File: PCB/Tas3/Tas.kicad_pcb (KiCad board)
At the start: 2 copper layers, 70 x 70 mm, 26 parts, among them J1 Shelly 1, J2 Conn_01x07, J3 USB-C, U1 MD8942, U2 Barcode, U3 CH340X, U4 ISL89410

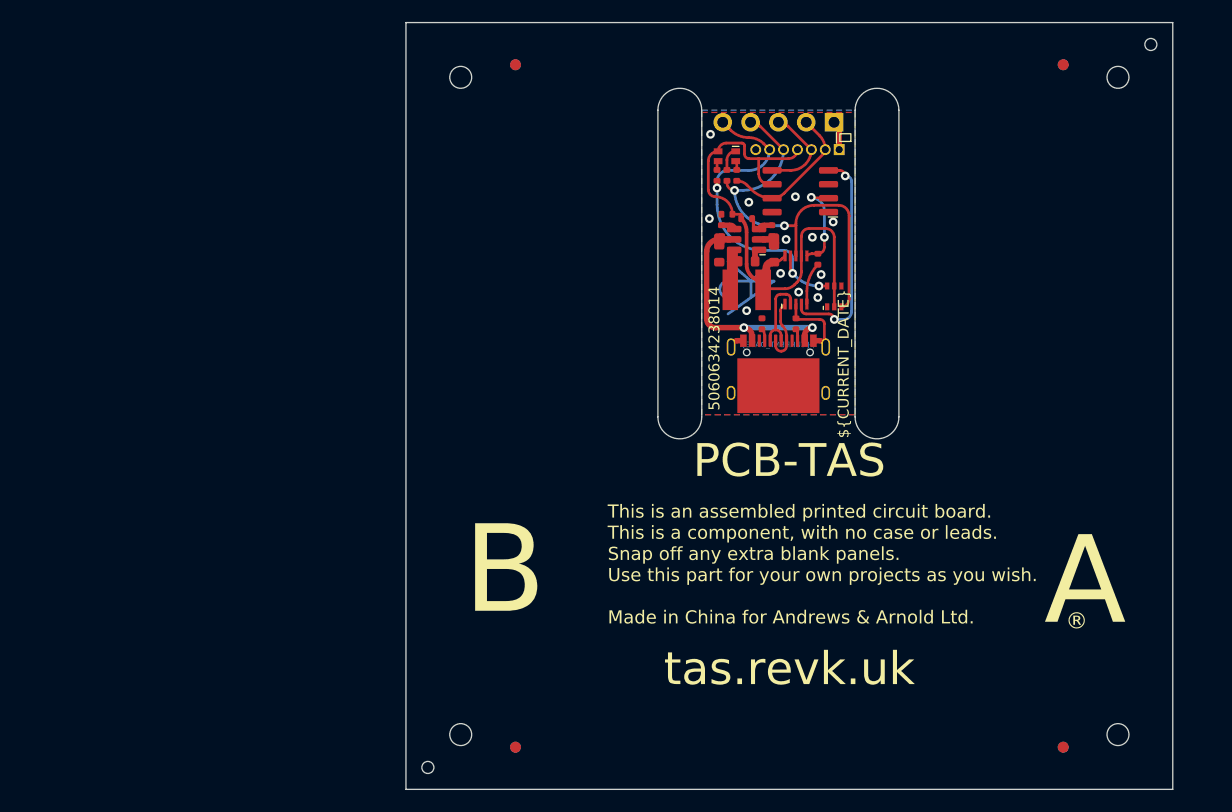
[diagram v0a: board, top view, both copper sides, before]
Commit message: VCUT
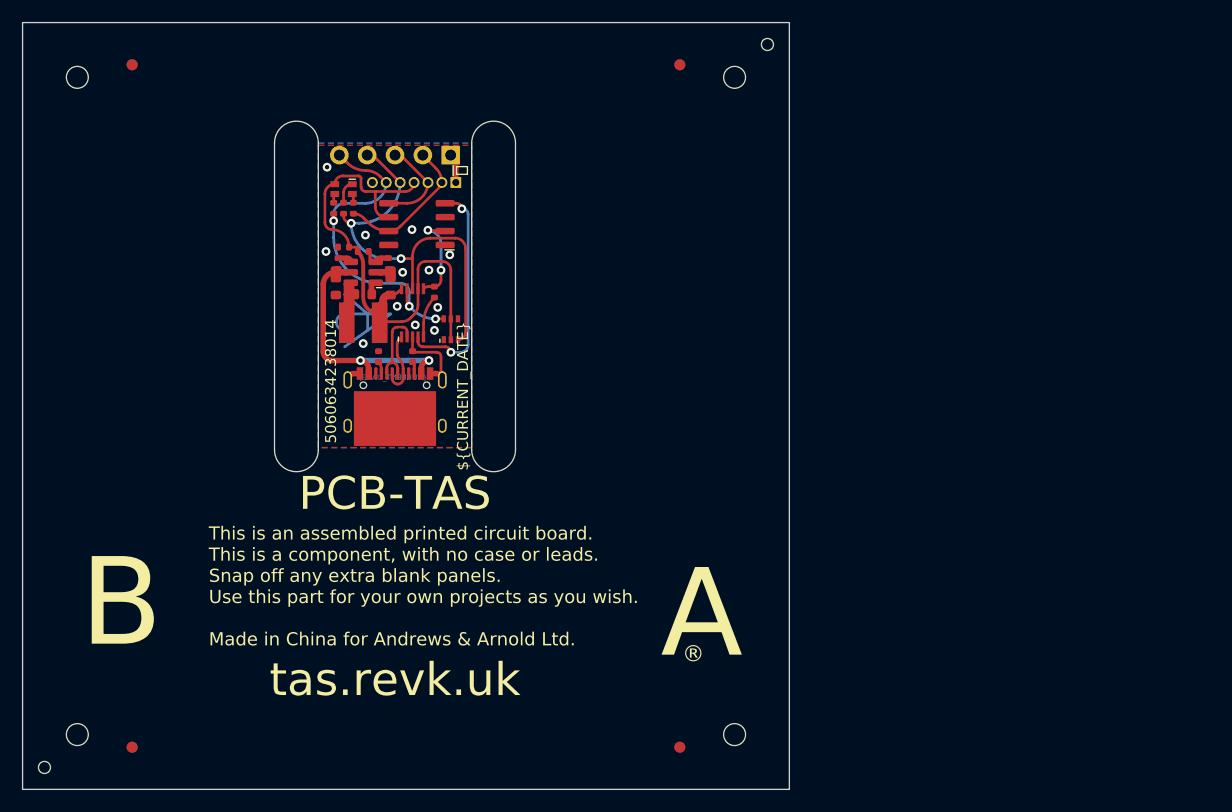
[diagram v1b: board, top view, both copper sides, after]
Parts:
- added V1: ~, RevK:VCUT70, F.Cu at (100.0, 68.9)
- added V2: ~, RevK:VCUT70, F.Cu at (100.0, 40.6)
- moved U2 36.0 mm to (117.5, 71.3)
- moved C5 35.1 mm to (94.3, 50.5)
- moved D5 35.1 mm to (94.3, 45.2)
- moved J2 35.1 mm to (100.7, 44.6)
- moved R10 35.1 mm to (93.8, 52.0)
- moved R11 35.1 mm to (94.3, 47.0)
- moved Art1 35.1 mm to (96.5, 56.6)
- moved Art2 35.1 mm to (99.0, 66.0)
- moved C1 35.1 mm to (93.6, 54.1)
- moved C6 35.1 mm to (98.6, 54.1)
- moved C7 35.1 mm to (96.1, 54.8)
- moved D1 35.1 mm to (104.1, 58.0)
- moved J1 35.1 mm to (99.0, 42.1)
- moved J3 35.1 mm to (99.0, 64.5)
- moved L2 35.1 mm to (96.1, 57.4)
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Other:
- board text added: "${TITLE}"
- board text removed: "2 Designs, 0.8mm, Black"
- board text removed: "PCB-TAS"
